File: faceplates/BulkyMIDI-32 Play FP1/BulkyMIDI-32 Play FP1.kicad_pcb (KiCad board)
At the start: 2 copper layers, 100 x 23.2 mm, 5 parts, among them M1 Mounting_Pin, M2 Mounting_Pin, M3 Mounting_Pin, M4 Mounting_Pin

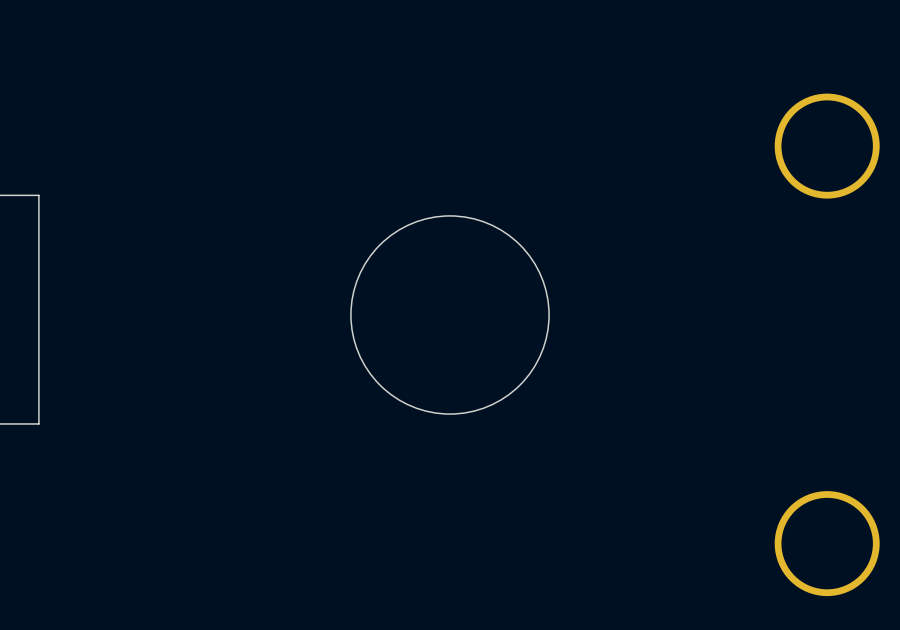
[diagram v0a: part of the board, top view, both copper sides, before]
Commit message: Build tweaks
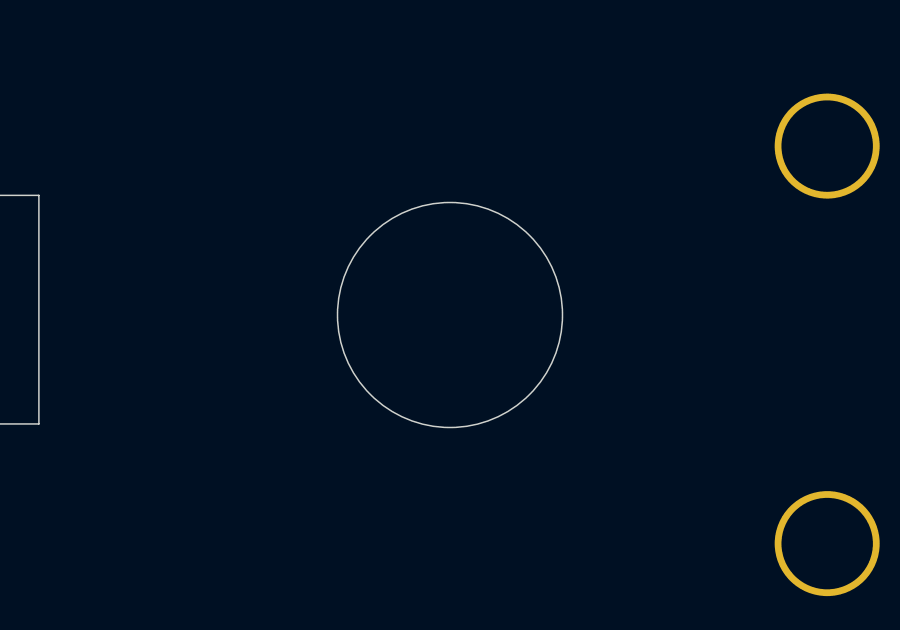
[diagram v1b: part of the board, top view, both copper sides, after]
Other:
- outline, holes or cut-outs redrawn
- board text added: "BulkyMIDI-32 Play FP1 (rev. B) github.com/tebl"
- board text removed: "BulkyMIDI-32 Play FP1 (rev. A) github.com/tebl"
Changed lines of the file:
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@@
   (gr_line (start 156.0887 117.5912) (end 156.0887 125.2112) (layer Edge.Cuts) (width 0.05))
   (gr_line (start 126.0913 117.5912) (end 156.0887 117.5912) (layer Edge.Cuts) (width 0.05))
-  (gr_circle (center 169.792 121.579) (end 173.094 121.579) (layer Edge.Cuts) (width 0.05))
-  (gr_text "BulkyMIDI-32\nPlay FP1 (rev. A)\ngithub.com/tebl" (at 94.1 122.849 270) (layer B.SilkS)
+  (gr_circle (center 169.792 121.579) (end 173.542 121.579) (layer Edge.Cuts) (width 0.05))
+  (gr_text "BulkyMIDI-32\nPlay FP1 (rev. B)\ngithub.com/tebl" (at 94.1 122.849 270) (layer B.SilkS)
     (effects (font (size 0.8 0.8) (thickness 0.1)) (justify mirror))
   )
